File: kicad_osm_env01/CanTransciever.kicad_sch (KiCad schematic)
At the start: 23 parts, among them U8 SN65HVD230

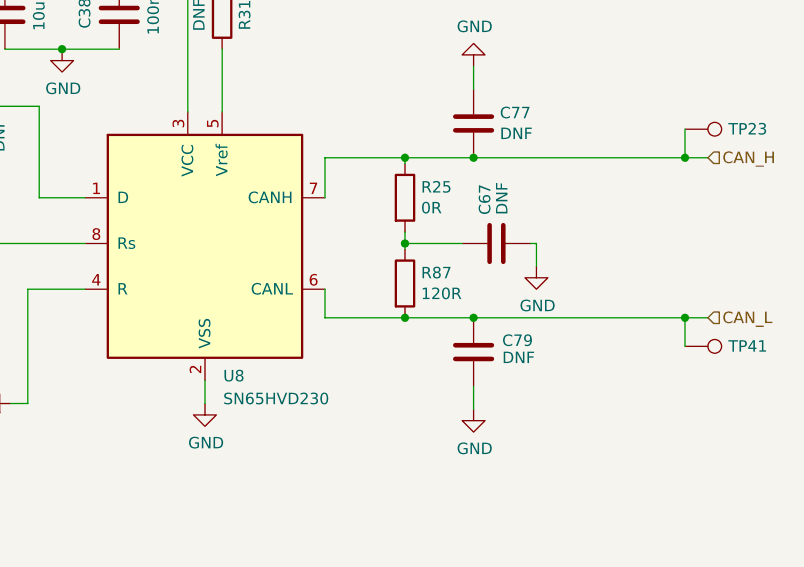
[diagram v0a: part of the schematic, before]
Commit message: added tracking to layout
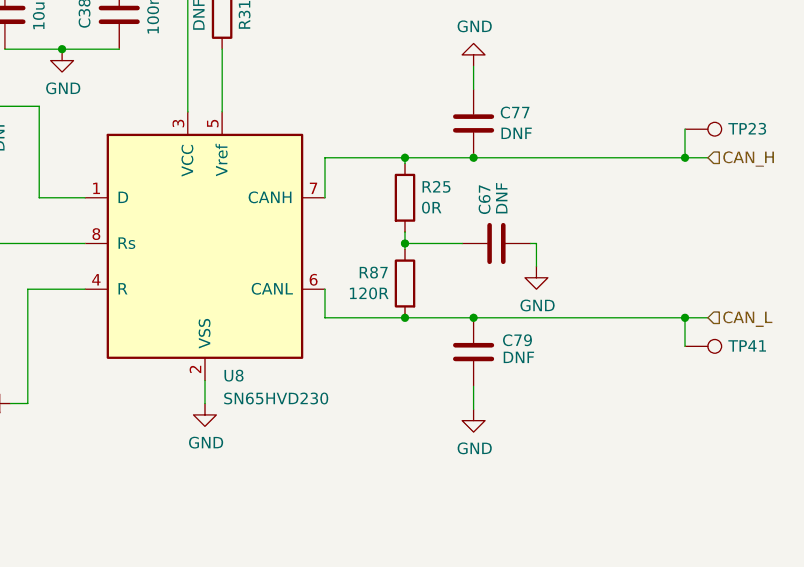
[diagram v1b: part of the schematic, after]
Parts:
- TP22, TP23, TP41, TP80, TP81: footprint TestPoint:TestPoint_THTPad_D1.0mm_Drill0.5mm -> TestPoint:TestPoint_Pad_D1.5mm
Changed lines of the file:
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@@
     )
   )
-  (symbol (lib_id "Device:R") (at 175.26 106.045 0) (unit 1)
-    (in_bom yes) (on_board yes) (dnp no)
-    (property "Reference" "R87" (at 177.038 104.8766 0)
-      (effects (font (size 1.27 1.27)) (justify left))
-    )
-    (property "Value" "120R" (at 177.038 107.188 0)
-      (effects (font (size 1.27 1.27)) (justify left))
-    )
-    (property "Footprint" "Resistor_SMD:R_0603_1608Metric" (at 173.482 106.045 90)
+  (symbol (lib_id "Device:R") (at 175.26 106.045 0) (mirror y) (unit 1)
+    (in_bom yes) (on_board yes) (dnp no)
+    (property "Reference" "R87" (at 173.482 104.8766 0)
+      (effects (font (size 1.27 1.27)) (justify left))
+    )
+    (property "Value" "120R" (at 173.482 107.188 0)
+      (effects (font (size 1.27 1.27)) (justify left))
+    )
+    (property "Footprint" "Resistor_SMD:R_0603_1608Metric" (at 177.038 106.045 90)
       (effects (font (size 1.27 1.27)) hide)
     )
@@
       (effects (font (size 1.27 1.27)) hide)
     )
-    (property "Footprint" "TestPoint:TestPoint_THTPad_D1.0mm_Drill0.5mm" (at 111.76 88.265 0)
+    (property "Footprint" "TestPoint:TestPoint_Pad_D1.5mm" (at 111.76 88.265 0)
       (effects (font (size 1.27 1.27)) hide)
     )
@@
       (effects (font (size 1.27 1.27)) hide)
     )
-    (property "Footprint" "TestPoint:TestPoint_THTPad_D1.0mm_Drill0.5mm" (at 117.475 122.555 0)
+    (property "Footprint" "TestPoint:TestPoint_Pad_D1.5mm" (at 117.475 122.555 0)
       (effects (font (size 1.27 1.27)) hide)
     )
@@
       (effects (font (size 1.27 1.27)) hide)
     )
-    (property "Footprint" "TestPoint:TestPoint_THTPad_D1.0mm_Drill0.5mm" (at 109.22 100.965 0)
+    (property "Footprint" "TestPoint:TestPoint_Pad_D1.5mm" (at 109.22 100.965 0)
       (effects (font (size 1.27 1.27)) hide)
     )
@@
       (effects (font (size 1.27 1.27)) hide)
     )
-    (property "Footprint" "TestPoint:TestPoint_THTPad_D1.0mm_Drill0.5mm" (at 206.375 93.98 0)
+    (property "Footprint" "TestPoint:TestPoint_Pad_D1.5mm" (at 206.375 93.98 0)
       (effects (font (size 1.27 1.27)) hide)
     )
@@
       (effects (font (size 1.27 1.27)) hide)
     )
-    (property "Footprint" "TestPoint:TestPoint_THTPad_D1.0mm_Drill0.5mm" (at 206.375 118.11 0)
-      (effects (font (size 1.27 1.27)) hide)
-    )
+    (property "Footprint" "TestPoint:TestPoint_Pad_D1.5mm" (at 206.375 118.11 0)
+      (effects (font (size 1.27 1.27)) hide)
+    )
